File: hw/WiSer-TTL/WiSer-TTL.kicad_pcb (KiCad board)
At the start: 4 copper layers, 28 x 29 mm, 62 parts, among them J1 USB_C_Receptacle_USB2.0, J2 Conn_01x02, J3 Conn_01x02, J4 Conn_01x02, J5 Conn_01x08, U1 USBLC6-2P6, U2 AP2112K-3.3TRG1, U3 ESP32-S2, Y1 40MHz

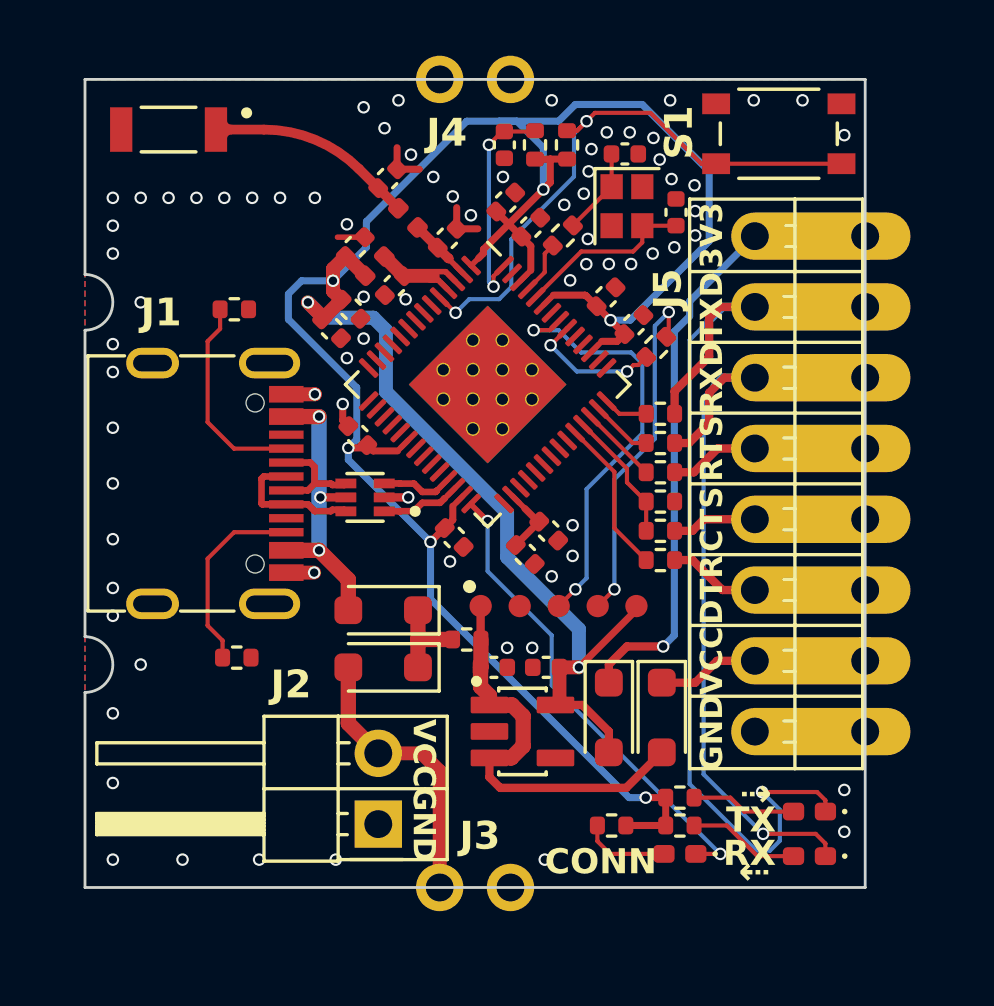
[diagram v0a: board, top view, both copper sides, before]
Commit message: Update hardware design files
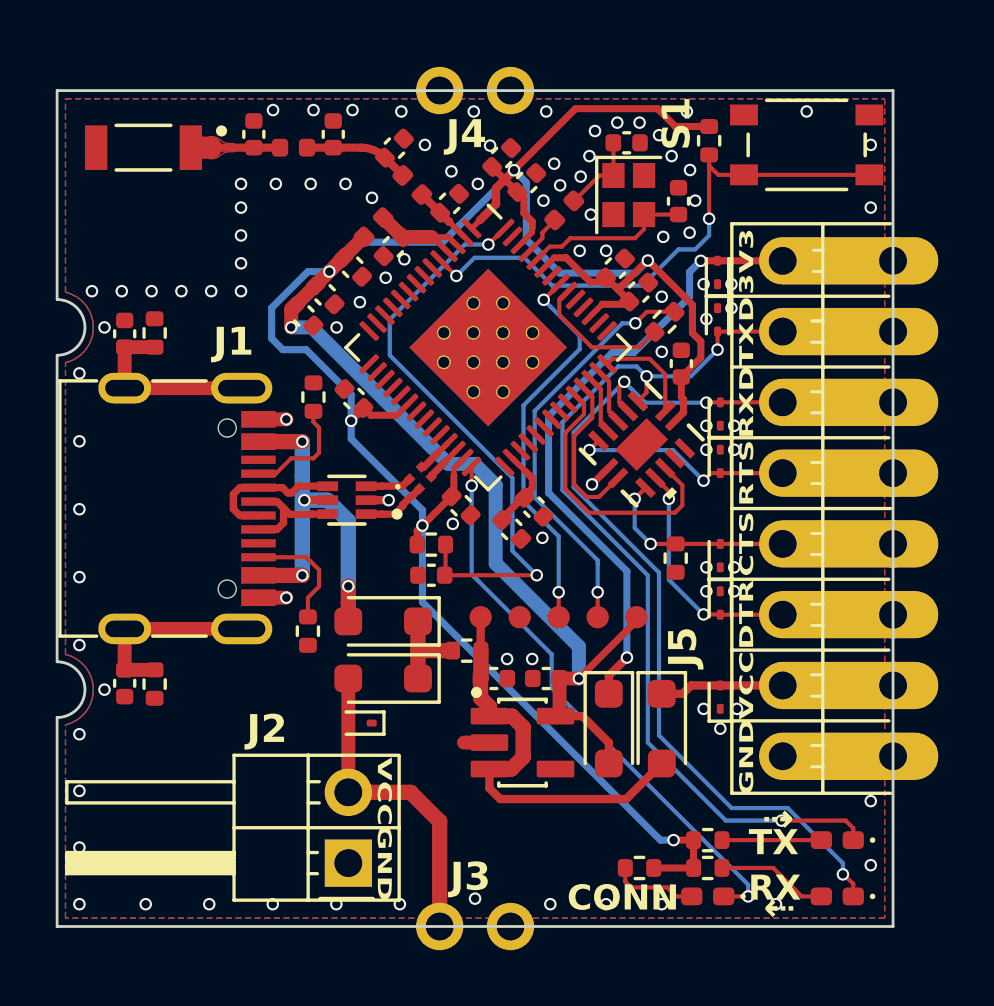
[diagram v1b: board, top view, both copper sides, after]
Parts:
- removed the C18 at (103.0, 82.3)
- removed the R10 at (110.7, 92.8)
- removed the R3 at (107.2, 82.2)
- removed the R5 at (110.7, 93.8)
- removed the R7 at (110.7, 88.6)
- removed the R8 at (110.7, 89.7)
- removed the R9 at (110.7, 90.7)
- added C1: 0.1u, Capacitor_SMD:C_0402_1005Metric, F.Cu at (91.4, 85.7)
- added C17: TBD, Capacitor_SMD:C_0402_1005Metric, F.Cu at (96.1, 78.6)
- added C19: TBD, Capacitor_SMD:C_0402_1005Metric, F.Cu at (98.9, 78.6)
- added C23: TBD, Capacitor_SMD:C_0402_1005Metric, F.Cu at (103.1, 81.0)
- added C24: 0.1u, Capacitor_SMD:C_0402_1005Metric, F.Cu at (111.4, 86.8)
- added C3: 0.1u, Capacitor_SMD:C_0402_1005Metric, F.Cu at (91.4, 98.3)
- added D1: ESD9B5.0ST5G, Diode_SMD:D_SOD-923, F.Cu at (99.9, 99.7)
- added D10: ESD9B5.0ST5G, Diode_SMD:D_SOD-923, F.Cu at (112.7, 85.2)
- added D11: ESD9B5.0ST5G, Diode_SMD:D_SOD-923, F.Cu at (112.8, 88.6)
- added D12: ESD9B5.0ST5G, Diode_SMD:D_SOD-923, F.Cu at (112.8, 90.3)
- added D13: ESD9B5.0ST5G, Diode_SMD:D_SOD-923, F.Cu at (112.8, 93.7)
- added D14: ESD9B5.0ST5G, Diode_SMD:D_SOD-923, F.Cu at (112.8, 95.4)
- added D15: ESD9B5.0ST5G, Diode_SMD:D_SOD-923, F.Cu at (112.8, 98.8)
- added D6: ESD9B3.3ST5G, Diode_SMD:D_SOD-923, F.Cu at (112.7, 83.5)
- added L2: L_Ferrite_Coupled_Small_1243, DLM0NSM900HY2D:FIL_DLM0NSM900HY2D, F.Cu at (102.0, 90.9)
- added L3: TBD, Inductor_SMD:L_0402_1005Metric, F.Cu at (97.5, 79.0)
- added L4: 24n, Inductor_SMD:L_0402_1005Metric, F.Cu at (107.2, 81.3)
- added R1: 330, Resistor_SMD:R_0402_1005Metric, F.Cu at (92.5, 85.7)
- added R2: 330, Resistor_SMD:R_0402_1005Metric, F.Cu at (92.5, 98.3)
- added U4: SN74LV6T17BQAR, SN74LV6T17BQAR:WQFN14_BQA_TEX, F.Cu at (110.0, 89.7)
- moved C22 15.7 mm to (102.4, 94.4), turned to 180 degrees
- moved R5 14.8 mm to (102.4, 93.3), turned to 0 degrees
- moved R8 5.10 mm to (112.4, 78.8), turned to -90 degrees
- moved R3 4.24 mm to (98.2, 88.0), turned to -90 degrees
- moved R4 2.72 mm to (98.0, 96.4), turned to 90 degrees
- moved R7 2.10 mm to (111.2, 93.8), turned to 90 degrees
- moved R10 1.82 mm to (112.3, 103.9)
- moved D9 1.82 mm to (112.3, 105.9)
- moved R9 1.82 mm to (112.3, 104.9)
- moved R11 1.82 mm to (109.9, 104.9)
- moved J2 1.77 mm to (99.5, 104.7)
- moved D7 1.76 mm to (117.0, 105.9)
- moved G2 1.62 mm to (93.8, 100.0)
- moved C7 1.61 mm to (105.0, 79.4)
- moved C9 1.61 mm to (105.9, 80.3)
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- renumbered C8 to C10, C9 to C11, C10 to C12, C11 to C13, C12 to C14, C13 to C15, C14 to C16, C15 to C18, C1 to C2, C16 to C20, C17 to C21, C19 to C22, C2 to C4, C3 to C5, C4 to C6, C5 to C7, C6 to C8, C7 to C9, D1 to D2, D2 to D3, D3 to D4, D4 to D5, D5 to D7, D6 to D8, D7 to D9, L2 to L5, R14 to R10, R15 to R11, R1 to R3, R2 to R4, R4 to R5, R11 to R7, R12 to R8, R13 to R9
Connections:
- C21 pad 1: Net-(C17-Pad1) -> Net-(C19-Pad1)
- D7 pad 1: /UART_RXD -> /TTL_RXD
- D8 pad 1: /UART_TXD -> /TTL_TXD
- J1 pad S1: unconnected-(J1-SHIELD-PadS1) -> Net-(J1-SHIELD)
- J5 pad 2: /UART_TXD -> /TTL_TXD
- J5 pad 3: /UART_RXD -> /TTL_RXD
- J5 pad 4: /UART_RTS -> /TTL_RTS
- J5 pad 5: /UART_CTS -> /TTL_CTS
- J5 pad 6: /UART_DTR -> /TTL_DTR
- L5 pad 1: Net-(C17-Pad1) -> Net-(C19-Pad1)
- R7 pad 1: Net-(U3-GPIO35) -> GND
- R7 pad 2: GND -> /TTL_CTS
- U3 pad 25: /USB- -> /USB_FIL-
- U3 pad 26: /USB+ -> /USB_FIL+
- U3 pad 38: Net-(U3-GPIO34) -> /UART_DTR
- U3 pad 39: Net-(U3-GPIO35) -> /UART_CTS
- U3 pad 40: Net-(U3-GPIO36) -> /UART_RTS
- U3 pad 41: Net-(U3-GPIO37) -> /UART_RXD
- U3 pad 42: Net-(U3-GPIO38) -> /UART_TXD
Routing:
- net /TTL_TXD: track 0.00 -> 32.8 mm, vias 0 -> 3
- net /TTL_RXD: track 0.00 -> 31.8 mm, vias 0 -> 3
- net /UART_TXD: track 33.7 -> 3.71 mm, vias 1 -> 0
- net /UART_RXD: track 26.0 -> 2.12 mm, vias 1 -> 0
- net Net-(J1-SHIELD): track 0.00 -> 13.4 mm
- net /CHIP_PU: track 7.93 -> 21.2 mm
- net /TTL_DTR: track 0.00 -> 8.46 mm, vias 0 -> 2
- net /TTL_RTS: track 0.00 -> 8.07 mm, vias 0 -> 2
- net /TTL_CTS: track 0.00 -> 7.12 mm, vias 0 -> 2
- net /UART_DTR: track 3.32 -> 10.0 mm
- net Net-(U3-GPIO34): track 5.63 -> 0.00 mm
- net +3V3: track 107.7 -> 112.8 mm
- net Net-(U3-GPIO35): track 4.75 -> 0.00 mm
- net Net-(C17-Pad1): track 7.48 -> 3.20 mm
- net Net-(C19-Pad1): track 0.00 -> 3.79 mm
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- added copper zone on F.Cu, net Net-(C17-Pad1)
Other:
- board size 28 x 29 mm -> 30 x 30 mm
- board text added: "Rev-1.2"
- board text removed: "Rev-1.1"
